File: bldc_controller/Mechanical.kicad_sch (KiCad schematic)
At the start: 5 parts

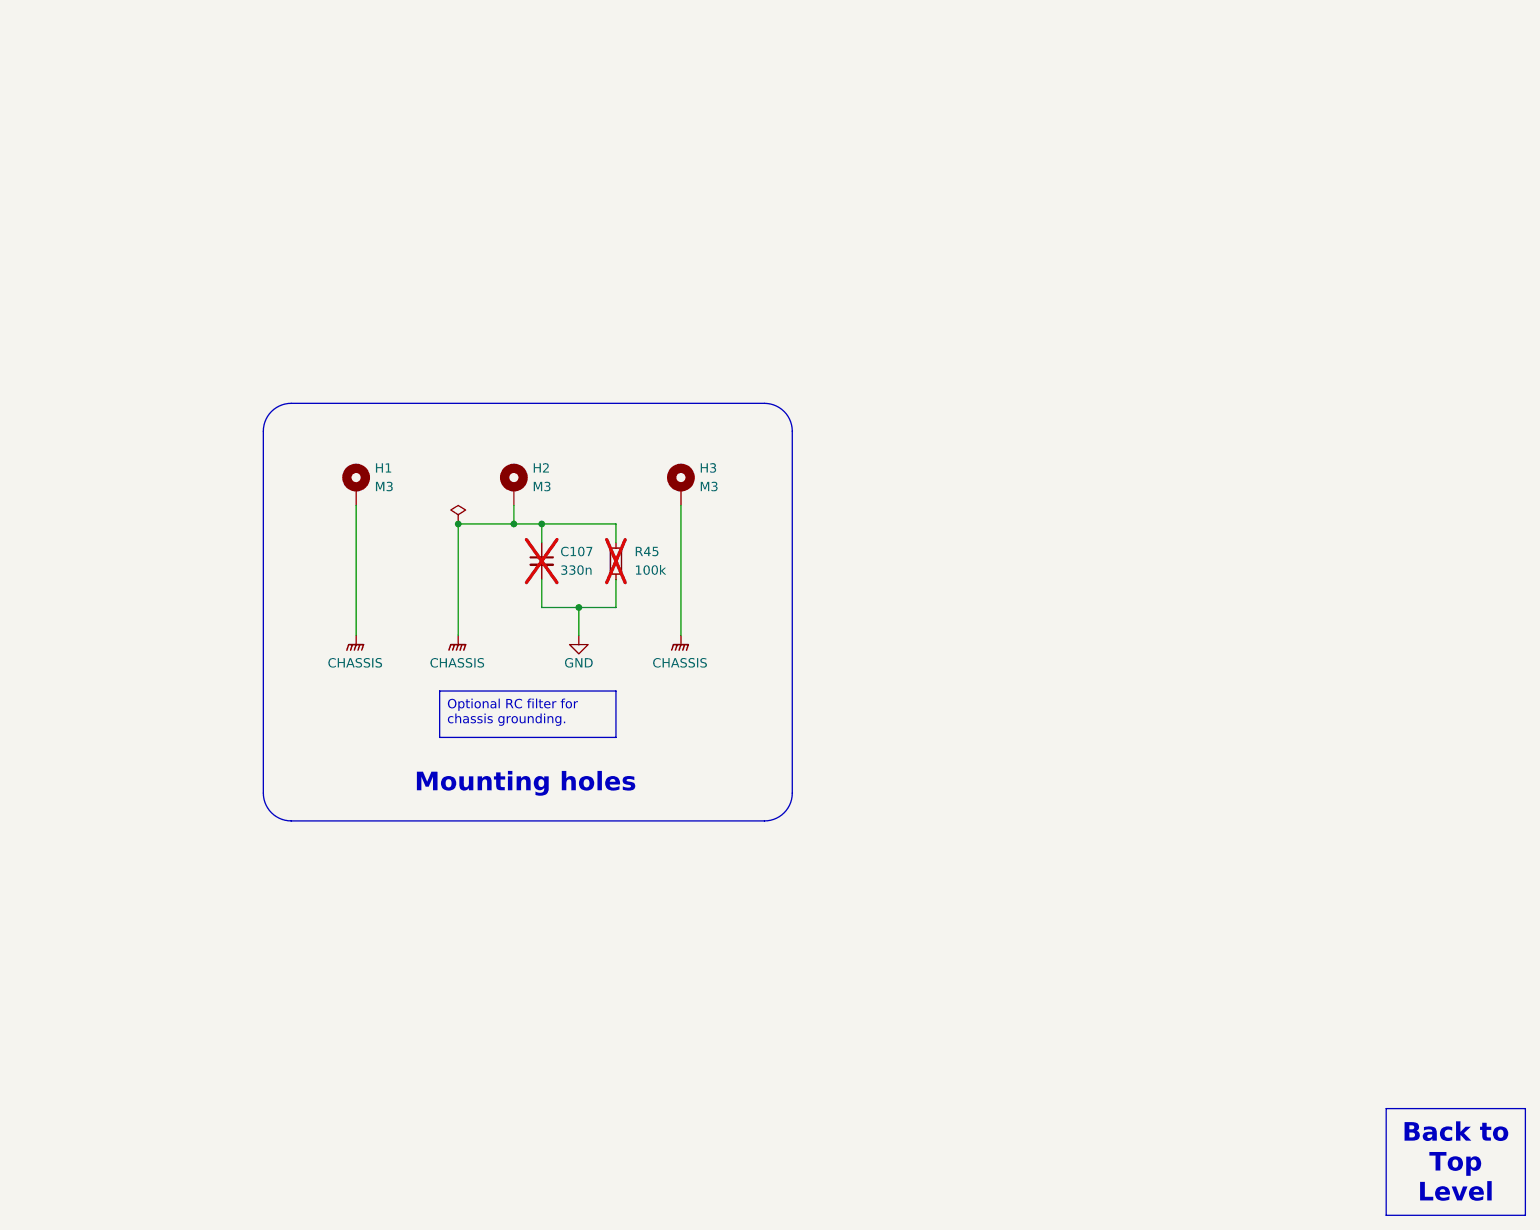
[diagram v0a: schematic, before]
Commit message: might have fixed net issue, added dxf and svgs
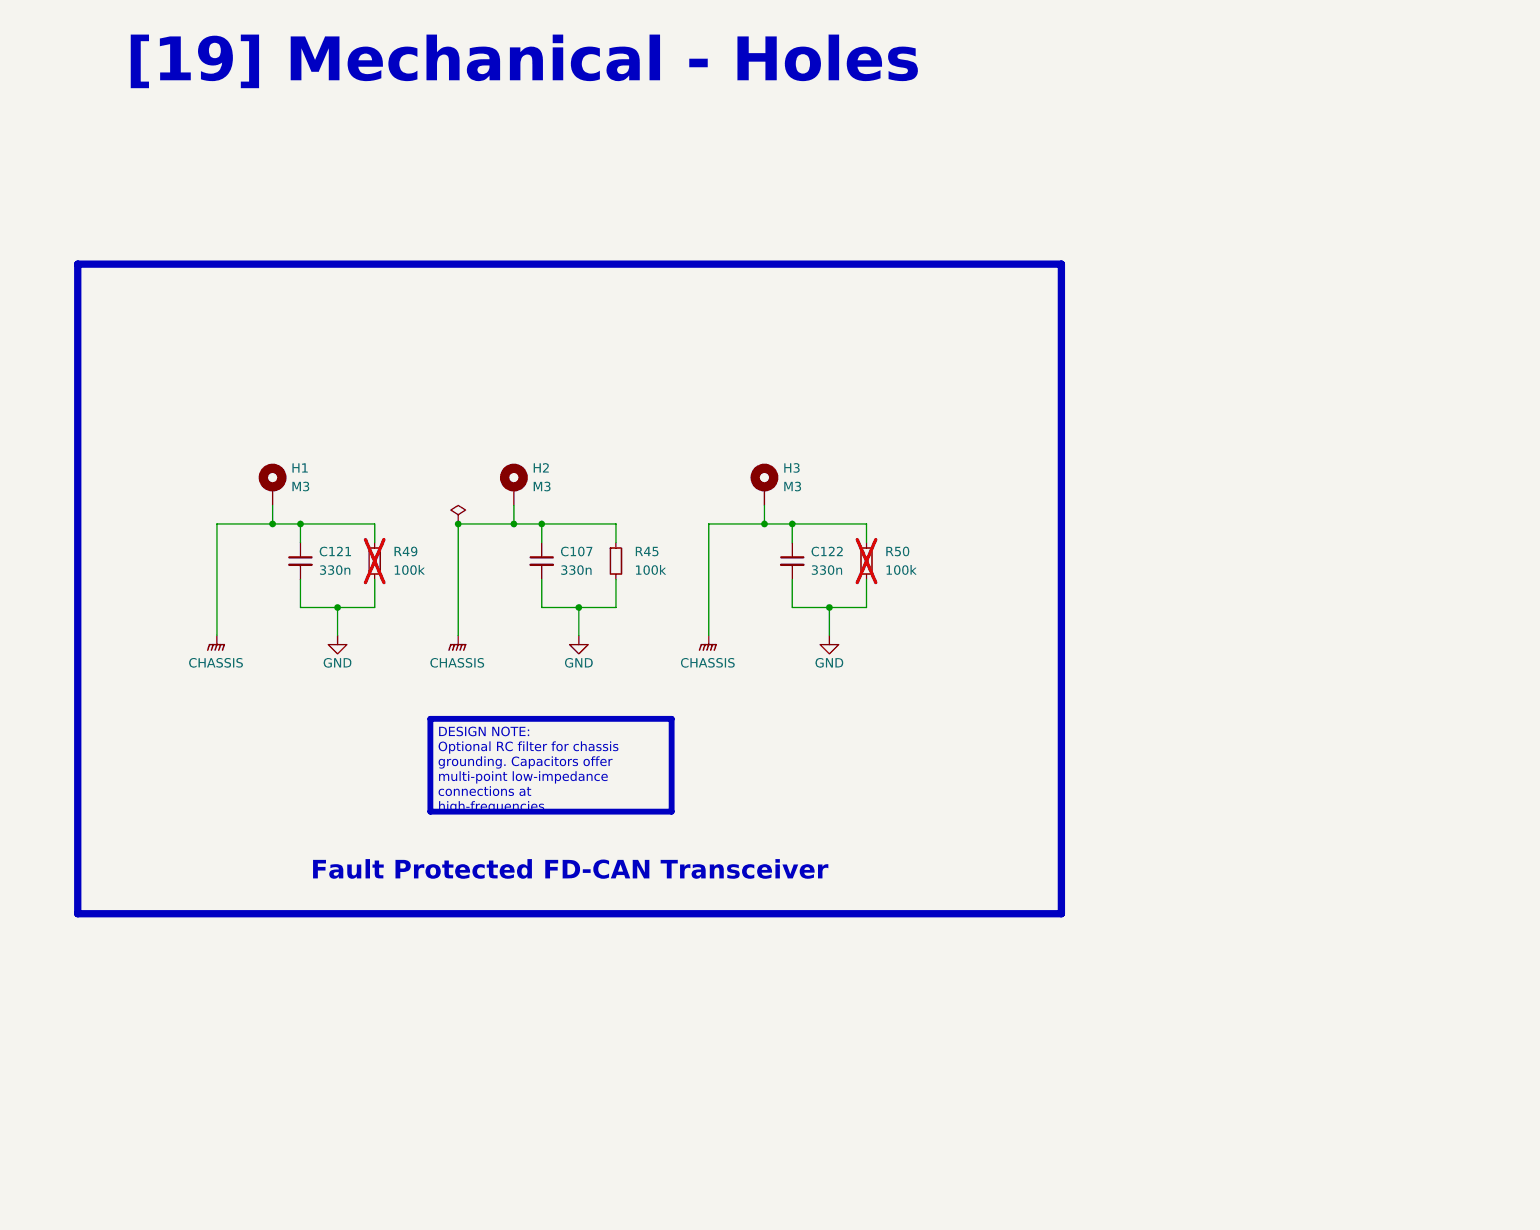
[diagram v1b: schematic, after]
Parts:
- added C121, C122: 330n, 0_capacitor_smd:C_0402_1005_DensityHigh, symbol Device:C_Small
- added R49, R50: 100k, 0_resistor_smd:R_0402_1005_DensityHigh, symbol Device:R_Small
- C107, R45: now fitted
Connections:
- net CHASSIS: now also C121.1, C122.1, R49.1, R50.1
- net GND: now also C121.2, C122.2, R49.2, R50.2
